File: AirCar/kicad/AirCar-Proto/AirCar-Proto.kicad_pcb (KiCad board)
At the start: 4 copper layers, 76.2 x 55.9 mm, 20 parts, among them J1 Conn_01x05, J3 Conn_01x06, J4 PJ-102A, SW2 SW_SPDT, U1 Pico, U2 LDL212PU50R, U3 TXU0104BQAR

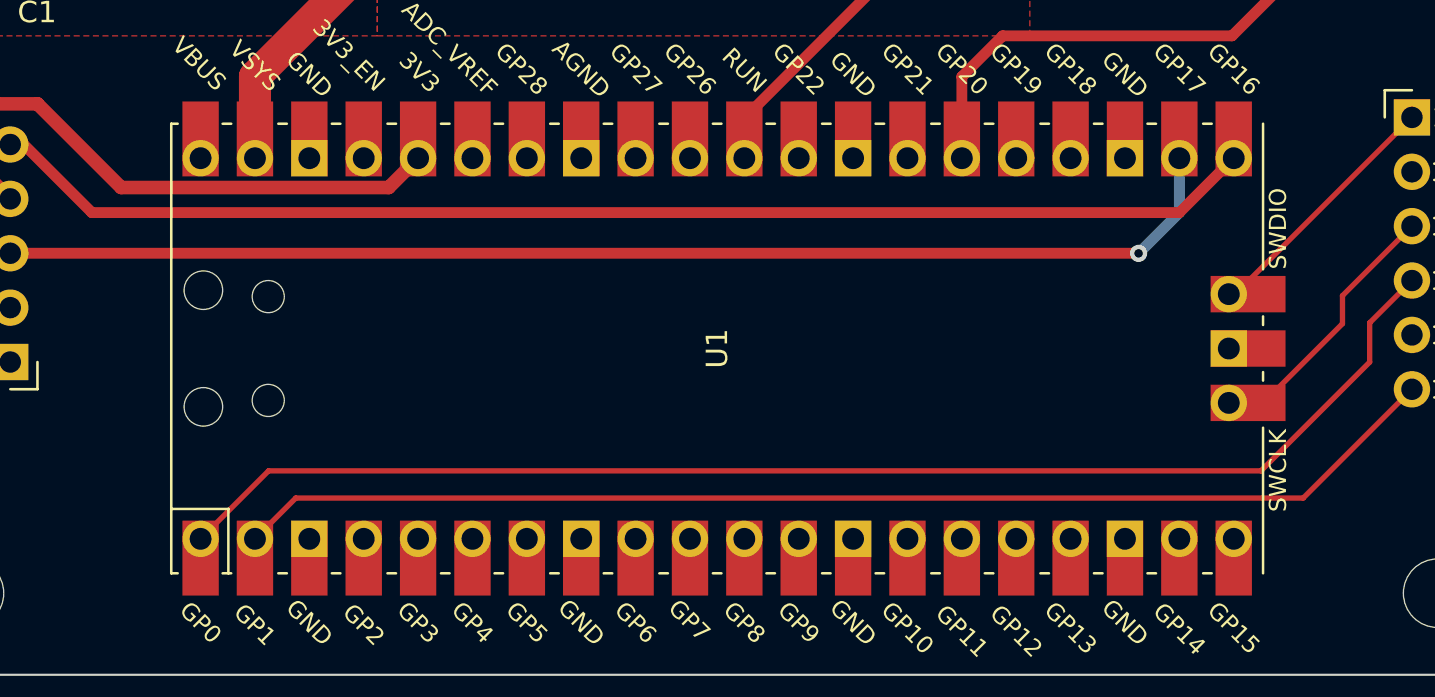
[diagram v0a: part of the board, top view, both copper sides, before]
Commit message: wip
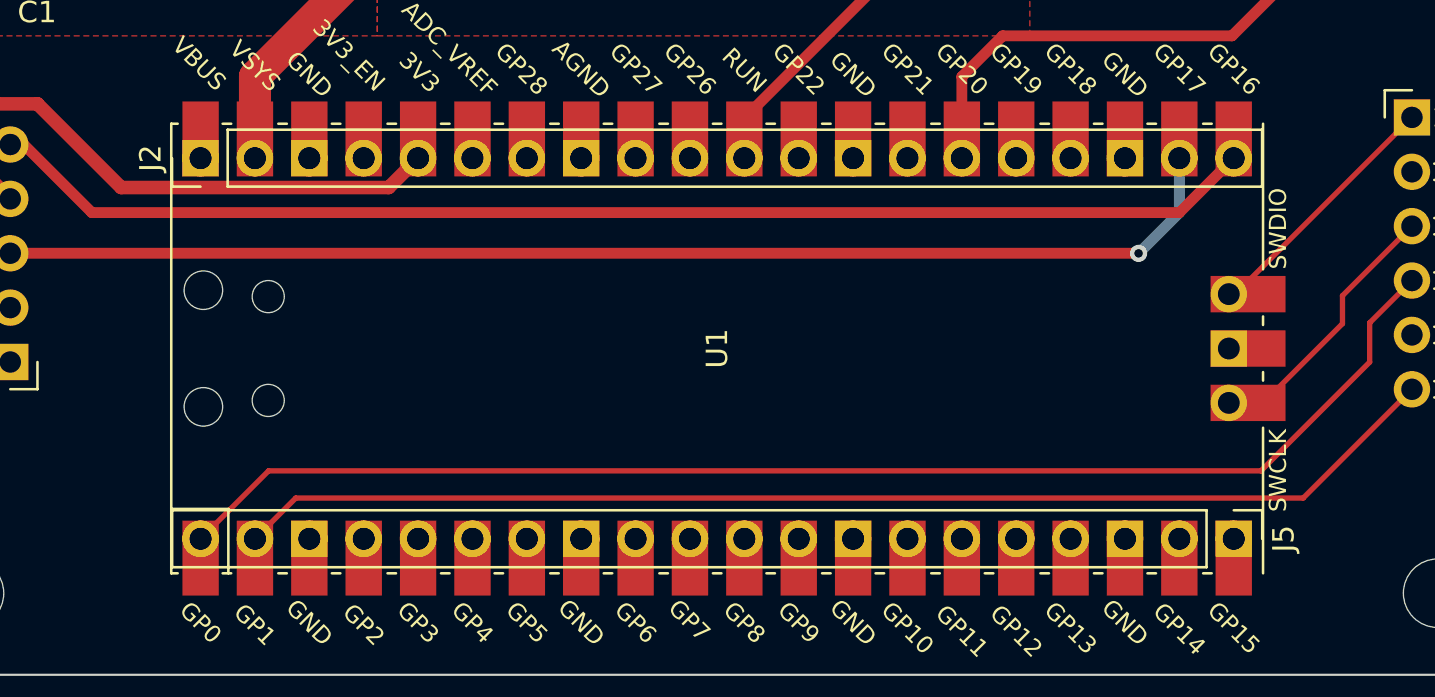
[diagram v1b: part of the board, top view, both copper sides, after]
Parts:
- added J2: Conn_01x20_Socket, Connector_PinHeader_2.54mm:PinHeader_1x20_P2.54mm_Vertical, F.Cu at (78.1, 133.3)
- added J5: Conn_01x20_Socket, Connector_PinHeader_2.54mm:PinHeader_1x20_P2.54mm_Vertical, F.Cu at (126.4, 151.1)
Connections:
- U1 pad 10: unconnected-(U1-GPIO7-Pad10) -> Net-(J5-Pin_11)
- U1 pad 11: unconnected-(U1-GPIO8-Pad11) -> Net-(J5-Pin_10)
- U1 pad 12: unconnected-(U1-GPIO9-Pad12) -> Net-(J5-Pin_9)
- U1 pad 13: unconnected-(U1-GND-Pad13) -> GND
- U1 pad 14: unconnected-(U1-GPIO10-Pad14) -> Net-(J5-Pin_7)
- U1 pad 15: unconnected-(U1-GPIO11-Pad15) -> Net-(J5-Pin_6)
- U1 pad 16: unconnected-(U1-GPIO12-Pad16) -> Net-(J5-Pin_5)
- U1 pad 17: unconnected-(U1-GPIO13-Pad17) -> Net-(J5-Pin_4)
- U1 pad 19: unconnected-(U1-GPIO14-Pad19) -> Net-(J5-Pin_2)
- U1 pad 20: unconnected-(U1-GPIO15-Pad20) -> Net-(J5-Pin_1)
- U1 pad 24: unconnected-(U1-GPIO18-Pad24) -> Net-(J2-Pin_17)
- U1 pad 25: unconnected-(U1-GPIO19-Pad25) -> Net-(J2-Pin_16)
- U1 pad 27: unconnected-(U1-GPIO21-Pad27) -> Net-(J2-Pin_14)
- U1 pad 29: unconnected-(U1-GPIO22-Pad29) -> Net-(J2-Pin_12)
- U1 pad 31: unconnected-(U1-GPIO26_ADC0-Pad31) -> Net-(J2-Pin_10)
- U1 pad 32: unconnected-(U1-GPIO27_ADC1-Pad32) -> Net-(J2-Pin_9)
- U1 pad 34: unconnected-(U1-GPIO28_ADC2-Pad34) -> Net-(J2-Pin_7)
- U1 pad 35: unconnected-(U1-ADC_VREF-Pad35) -> Net-(J2-Pin_6)
- U1 pad 37: unconnected-(U1-3V3_EN-Pad37) -> Net-(J2-Pin_4)
- U1 pad 4: unconnected-(U1-GPIO2-Pad4) -> Net-(J5-Pin_17)
- U1 pad 40: unconnected-(U1-VBUS-Pad40) -> Net-(J2-Pin_1)
- U1 pad 5: unconnected-(U1-GPIO3-Pad5) -> Net-(J5-Pin_16)
- U1 pad 6: unconnected-(U1-GPIO4-Pad6) -> Net-(J5-Pin_15)
- U1 pad 7: unconnected-(U1-GPIO5-Pad7) -> Net-(J5-Pin_14)
- U1 pad 9: unconnected-(U1-GPIO6-Pad9) -> Net-(J5-Pin_12)
